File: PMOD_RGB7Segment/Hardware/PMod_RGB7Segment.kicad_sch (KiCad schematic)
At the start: 1 part, among them J1 Conn_02x06_Counter_Clockwise

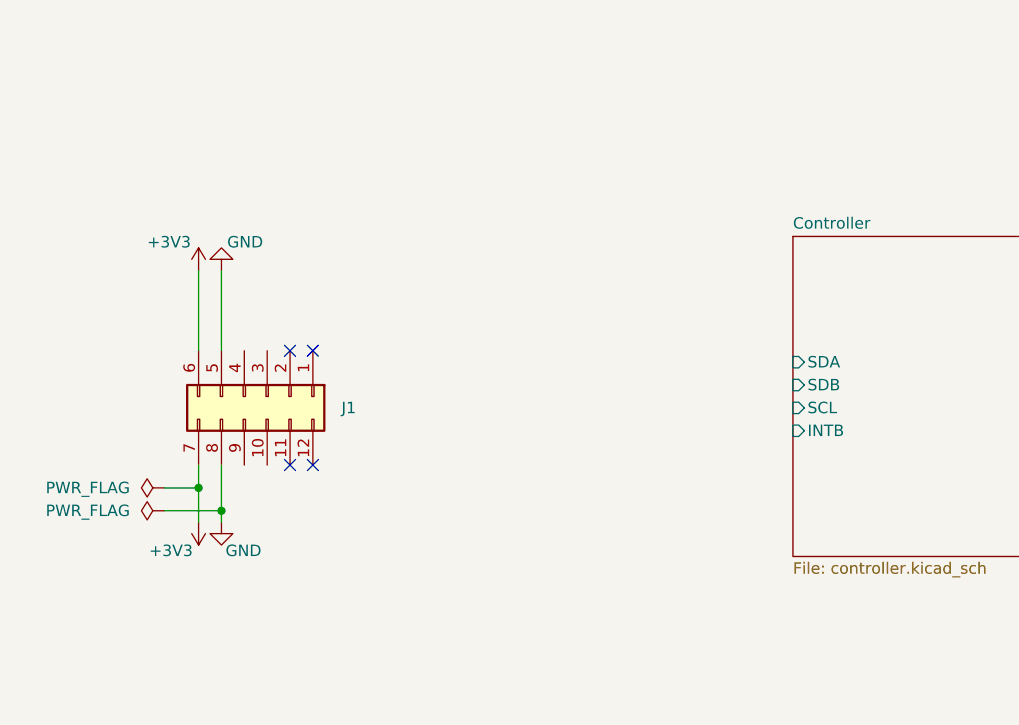
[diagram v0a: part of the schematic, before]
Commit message: start mapping out locations on PCB
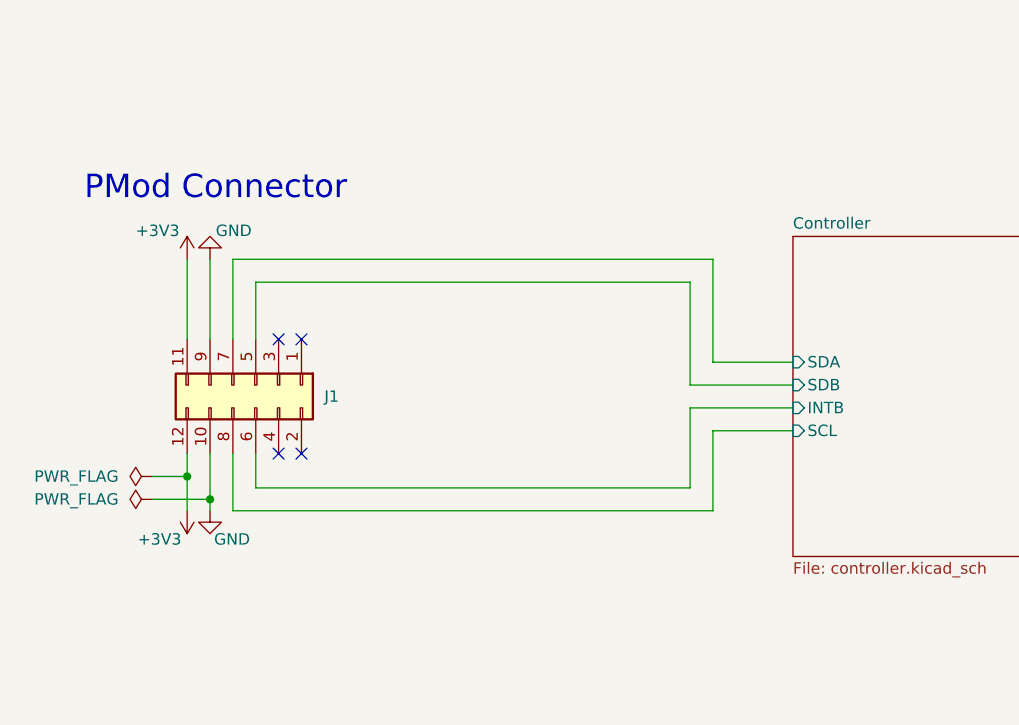
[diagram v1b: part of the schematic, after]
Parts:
- removed J1: Conn_02x06_Counter_Clockwise, Connector_PinHeader_2.54mm:PinHeader_2x06_P2.54mm_Vertical, symbol Connector_Generic:Conn_02x06_Counter_Clockwise
- added J1: Conn_02x06_Odd_Even, Connector_PinHeader_2.54mm:PinHeader_2x06_P2.54mm_Vertical, symbol Connector_Generic:Conn_02x06_Odd_Even
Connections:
- net +3V3: now also J1.11 (Pin_11), J1.12 (Pin_12)
- net Controller/INTB: now also J1.6 (Pin_6)
- net Controller/SCL: now also J1.8 (Pin_8)
- net Controller/SDA: now also J1.7 (Pin_7)
- net Controller/SDB: now also J1.5 (Pin_5)
- net GND: now also J1.10 (Pin_10), J1.9 (Pin_9)
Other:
- note added: "PMod Connector"
- company: (none) -> James Horton
- title: (none) -> PMod RGB & Segment Display
